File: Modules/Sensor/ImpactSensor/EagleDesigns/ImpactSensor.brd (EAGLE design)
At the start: 100 x 80 mm, 7 parts

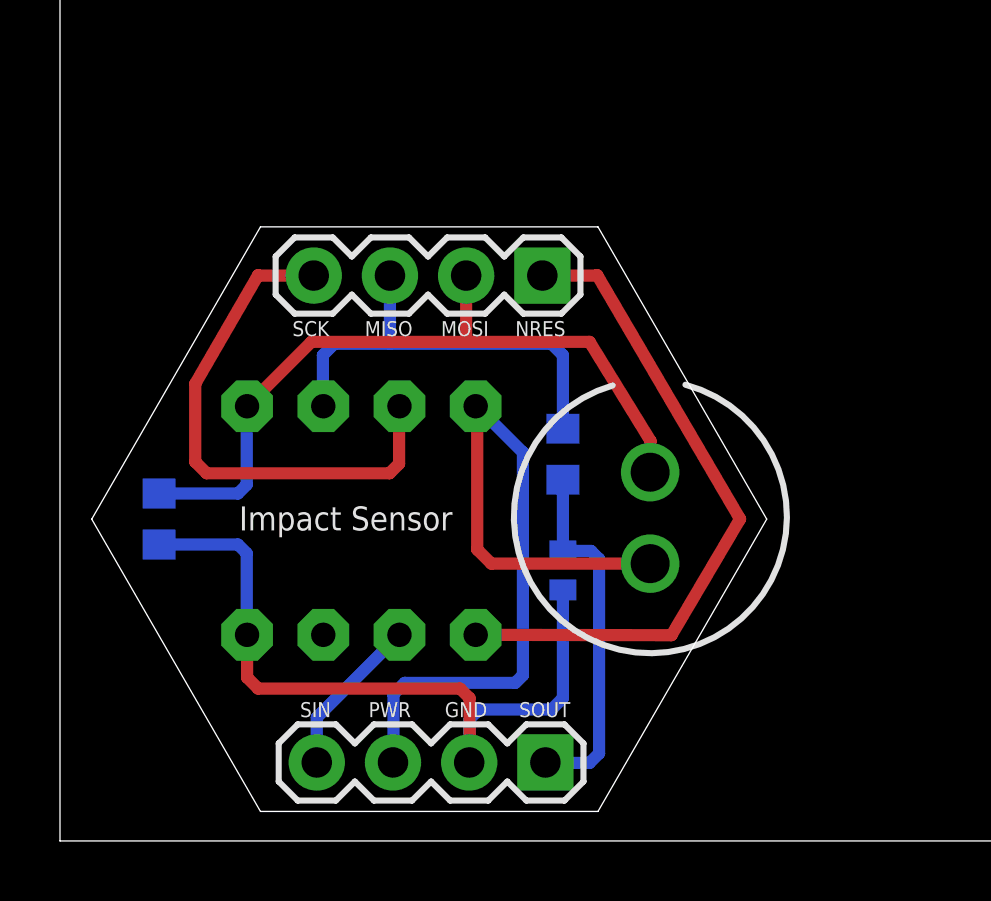
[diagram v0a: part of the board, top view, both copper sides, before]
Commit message: re-organized files after Merge
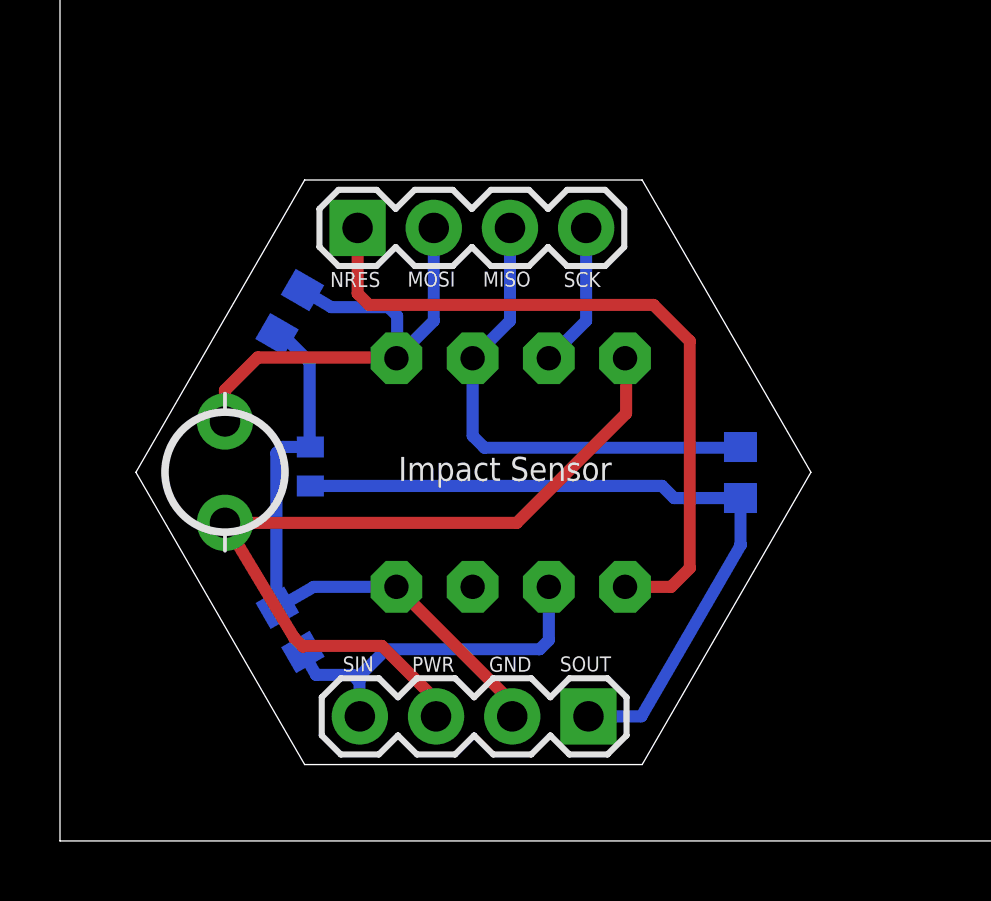
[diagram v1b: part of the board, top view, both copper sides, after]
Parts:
- removed CON, PROG: (no value), SparkFun-Connectors:1X04
- removed U: TINY85-20-DIP, SparkFun-DigitalIC:DIP08
- removed V: CM4400, sensor-comus-group:CM4400
- added JP1, JP2: (no value), SparkFun-Connectors:1X04
- added R3: 4.7K, adafruit:R0603
- added TILT1: TILT-AT407, SparkFun-Electromechanical:TILT-AT407
- added U2: TINY85-20-DIP, SparkFun-DigitalIC:DIP08
- R1: value 330K -> 1M
- R2: value 4.7K -> 330K
- moved R2 10.3 mm to (7.66, 17.6), turned to 120 degrees
- moved C1 9.11 mm to (8.34, 12.5), turned to 270 degrees
- moved R1 5.72 mm to (7.67, 7.04), turned to 240 degrees
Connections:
- net 1X3SIN: now also JP1.4, R1.2, U2.2; no longer CON.4, U.2
- net 1X3SOUT: now also JP1.1, R3.1; no longer CON.1, R2.1
- net GND: now also JP1.2, R2.1, U2.4; no longer CON.2, U.4
- net NRES: now also JP2.1, U2.1; no longer PROG.1, U.1
- net OUT(MISO): now also JP2.3, R3.2, U2.6; no longer PROG.3, R2.2, U.6
- net SCK: now also JP2.4, U2.7; no longer PROG.4, U.7
- net SENSOR(MOSI): now also JP2.2, R2.2, TILT1.P$2, U2.5; no longer PROG.2, R1.2, U.5, V.2
- net VCC: now also JP1.3, TILT1.P$1, U2.8; no longer CON.3, U.8, V.1
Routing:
- net SCK: track 17.7 -> 4.86 mm
- net 1X3SOUT: track 12.1 -> 24.4 mm
- net SENSOR(MOSI): track 25.1 -> 16.9 mm
- net 1X3SIN: track 5.40 -> 12.3 mm
- net GND: track 25.5 -> 20.8 mm
- net OUT(MISO): track 14.8 -> 16.6 mm
- net NRES: track 22.3 -> 23.9 mm
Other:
- outline, holes or cut-outs redrawn
